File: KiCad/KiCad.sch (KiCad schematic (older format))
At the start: 14 parts, among them P1 Power, P2 Analog, P3 Digital, P4 Digital

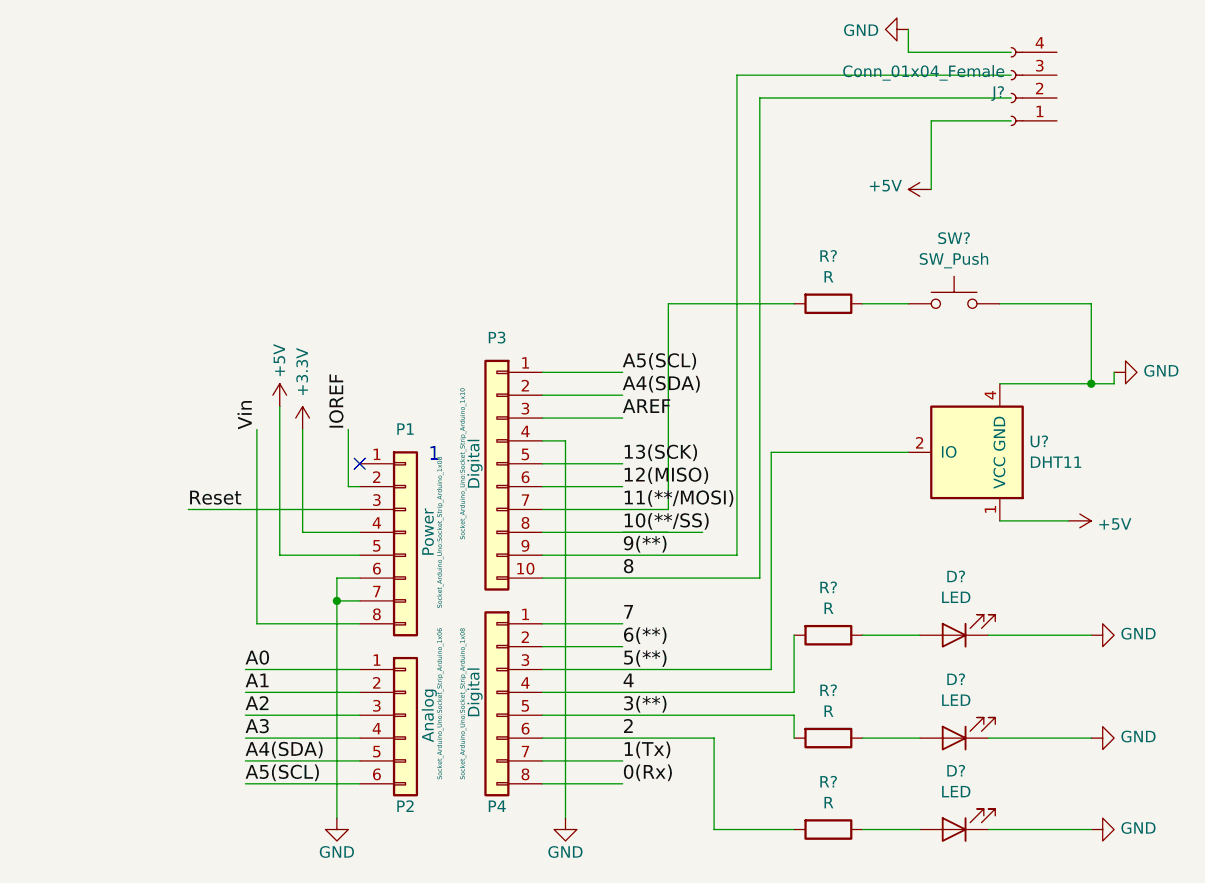
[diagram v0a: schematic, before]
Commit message: Aggiunta potenziometro
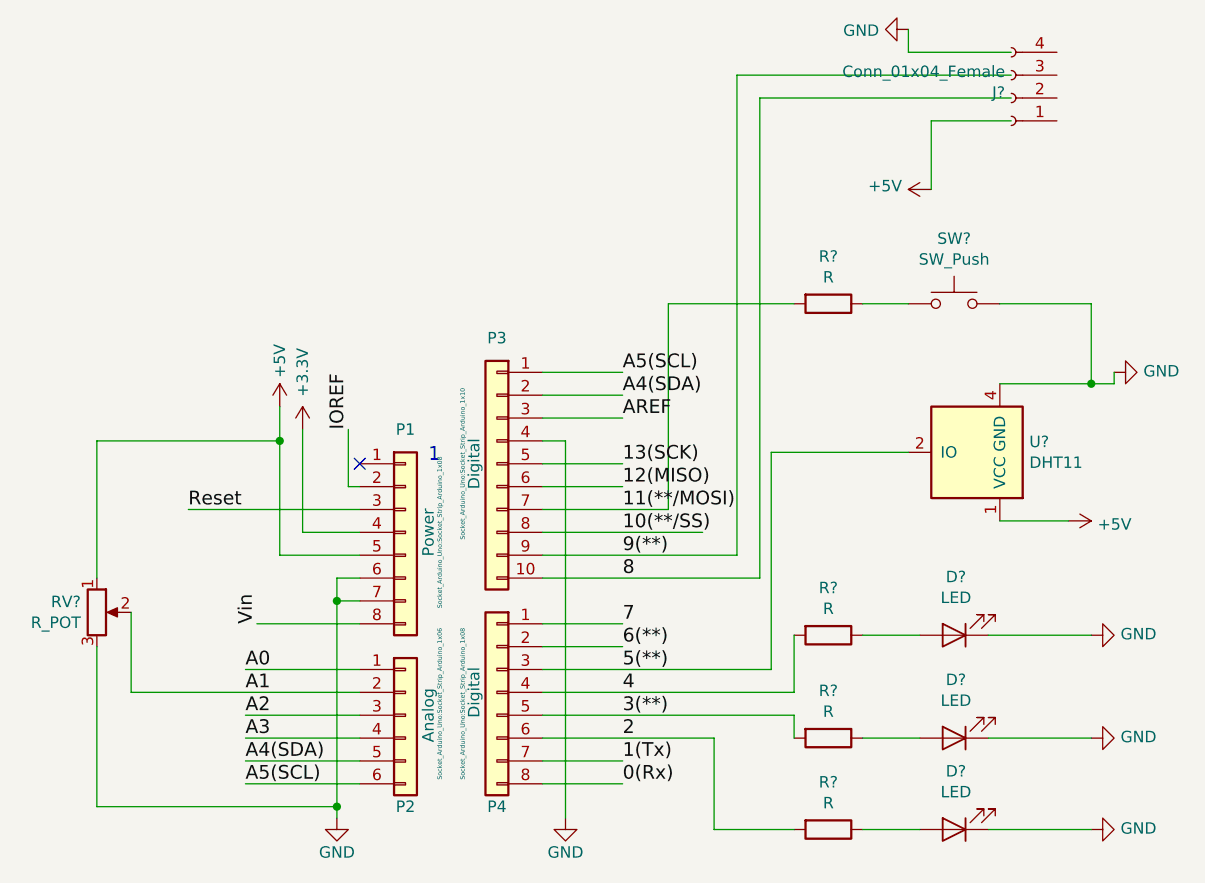
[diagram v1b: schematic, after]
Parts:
- added RV?: R_POT, symbol Device:R_POT
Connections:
- wire segments 68 -> 73
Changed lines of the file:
@@
 Comment4 ""
 $EndDescr
-Text Label 4750 3100 1    60   ~ 0
+Text Label 4750 3950 1    60   ~ 0
 Vin
 Text Label 5150 3100 1    60   ~ 0
@@
 Connection ~ 5100 3850
 Wire Wire Line
-	4750 3950 4750 3100
-Wire Wire Line
-	4850 3650 4850 3000
+	4850 3650 4850 3150
 Wire Wire Line
 	4950 3550 4950 3100
-Wire Wire Line
-	5200 4150 4700 4150
-Wire Wire Line
-	5200 4250 4700 4250
 Wire Wire Line
 	5200 4350 4700 4350
@@
 	5100 3750 5100 3850
 Wire Wire Line
-	5100 3850 5100 4800
+	5100 3850 5100 4750
 Wire Wire Line
 	5200 3450 4450 3450
@@
 $EndComp
 Wire Wire Line
+	8000 2900 8400 2900
+Wire Wire Line
+	7100 2550 6550 2550
+Wire Wire Line
+	6550 2550 6550 3450
+Wire Wire Line
+	6000 3450 6550 3450
+Wire Wire Line
+	7400 2550 7600 2550
+Wire Wire Line
 	6000 3550 6700 3550
-Wire Wire Line
-	8000 2900 8400 2900
-Wire Wire Line
-	7100 2550 6550 2550
-Wire Wire Line
-	6550 2550 6550 3450
-Wire Wire Line
-	6000 3450 6550 3450
-Wire Wire Line
-	6550 3550 6350 3550
-Wire Wire Line
-	7400 2550 7600 2550
+$Comp
+L Device:R_POT RV?
+U 1 1 5C86709E
+P 4050 3900
+F 0 "RV?" H 3980 3946 50  0000 R CNN
+F 1 "R_POT" H 3980 3855 50  0000 R CNN
+F 2 "" H 4050 3900 50  0001 C CNN
+F 3 "~" H 4050 3900 50  0001 C CNN
+	1    4050 3900
+	1    0    0    -1
+$EndComp
+Wire Wire Line
+	5200 4150 4700 4150
+Wire Wire Line
+	4050 3750 4050 3150
+Wire Wire Line
+	4050 3150 4850 3150
+Connection ~ 4850 3150
+Wire Wire Line
+	4850 3150 4850 3000
+Wire Wire Line
+	4200 3900 4200 4250
+Wire Wire Line
+	4200 4250 5200 4250
+Wire Wire Line
+	4050 4050 4050 4750
+Wire Wire Line
+	4050 4750 5100 4750
+Connection ~ 5100 4750
+Wire Wire Line
+	5100 4750 5100 4800
 $EndSCHEMATC
